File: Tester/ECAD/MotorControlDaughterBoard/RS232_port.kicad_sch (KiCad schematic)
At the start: 7 parts, among them J6 DB9_Male, U1 SP3243E

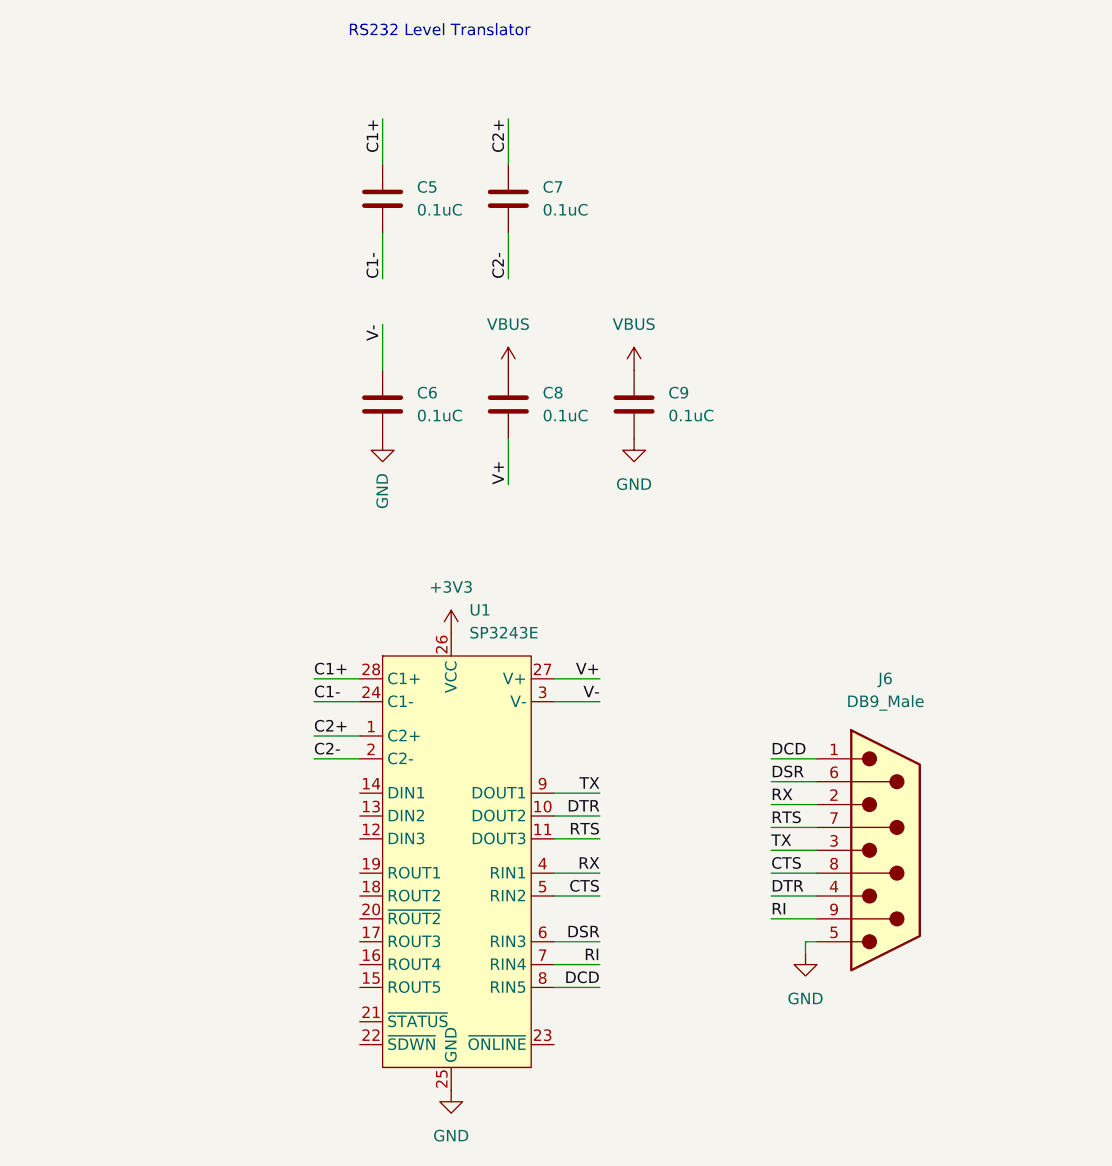
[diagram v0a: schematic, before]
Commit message: Progressed ECAD
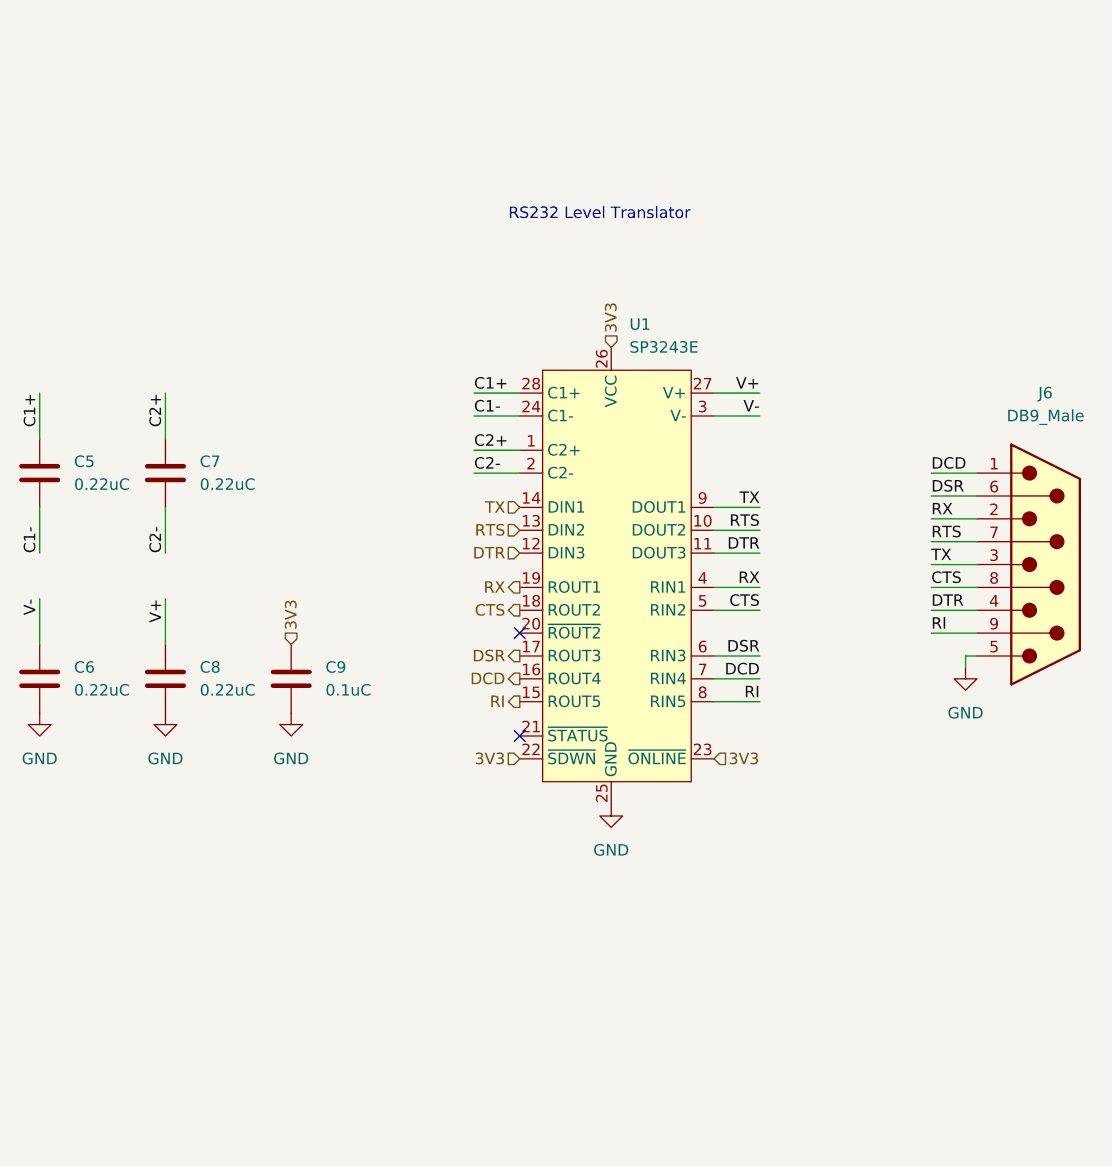
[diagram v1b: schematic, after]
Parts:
- C5, C6, C7, C8: value 0.1uC -> 0.22uC; Manufacturer Part Number CC0805KRX7R8BB104 -> C2012X7R1E224KT0H0N
- J6: Manufacturer Part Number D-DMR009PM-D002 -> DT00151-H1A2-4F
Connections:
- net +3V3 is gone; now on net 3V3: U1.26 (VCC)
- net CTS: now also U1.18 (ROUT2)
- net DCD: now also U1.16 (ROUT4), U1.7 (RIN4); no longer U1.8 (RIN5)
- net DSR: now also U1.17 (ROUT3)
- net DTR: now also U1.11 (DOUT3), U1.12 (DIN3); no longer U1.10 (DOUT2)
- net GND: now also C8.1
- net RI: now also U1.15 (ROUT5), U1.8 (RIN5); no longer U1.7 (RIN4)
- net RTS: now also U1.10 (DOUT2), U1.13 (DIN2); no longer U1.11 (DOUT3)
- net RX: now also U1.19 (ROUT1)
- net TX: now also U1.14 (DIN1)
- net V+: now also C8.2; no longer C8.1
- net 3V3: now reaches U1.22 (~{SDWN})
- net 3V3: now also C9.2, U1.23 (~{ONLINE})
- removed net VBUS: C8.2, C9.2
- no-connect marks 0 -> 2
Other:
- moved on the sheet: C5, C6, C7, C8, C9, J6, U1
